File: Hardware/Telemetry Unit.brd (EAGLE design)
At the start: 50.8 x 63.5 mm, 56 parts, among them IC1 MEGA128-A, IC2 FT232RL, J2 503182-1852, J3 10118193-0001LF, Q1 10MHz, U1 MPL3115A2, U2 AP65111A, U3 LSM6DS3

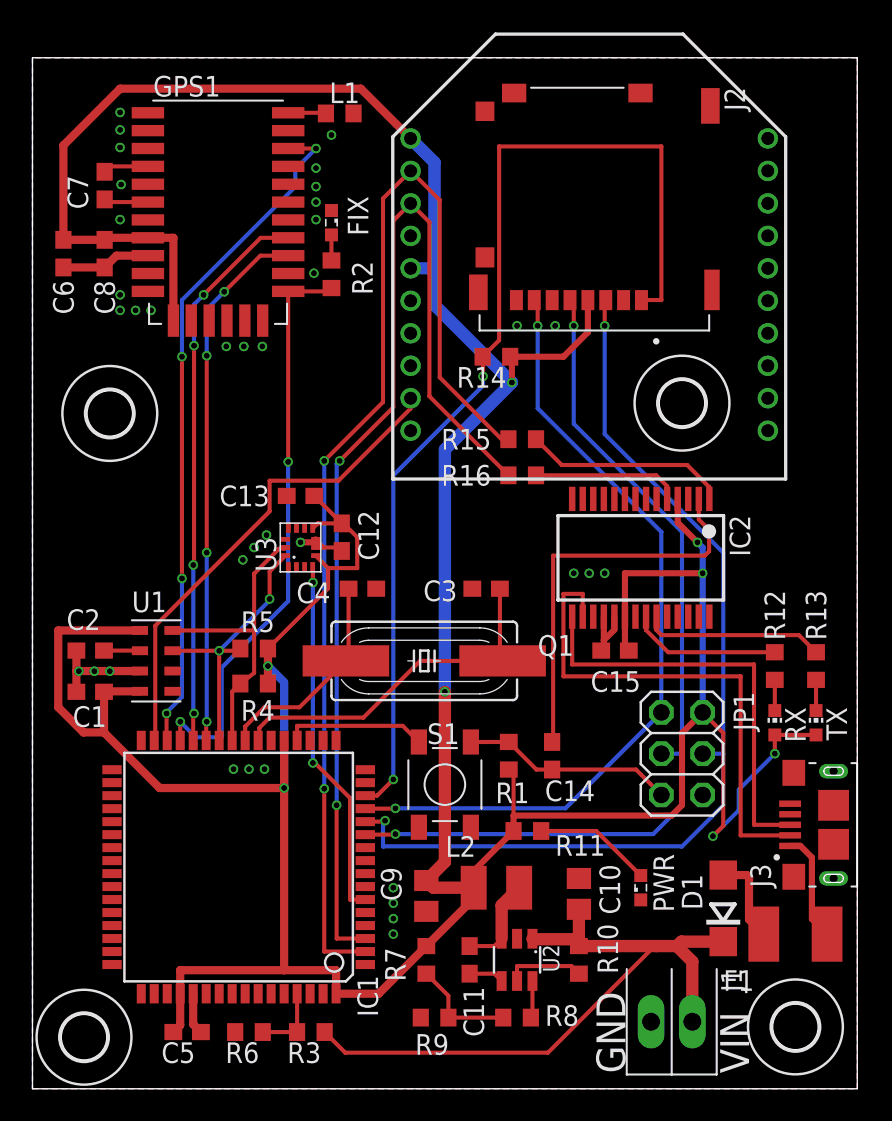
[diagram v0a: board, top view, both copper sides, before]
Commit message: Most minor updates and some rerouting
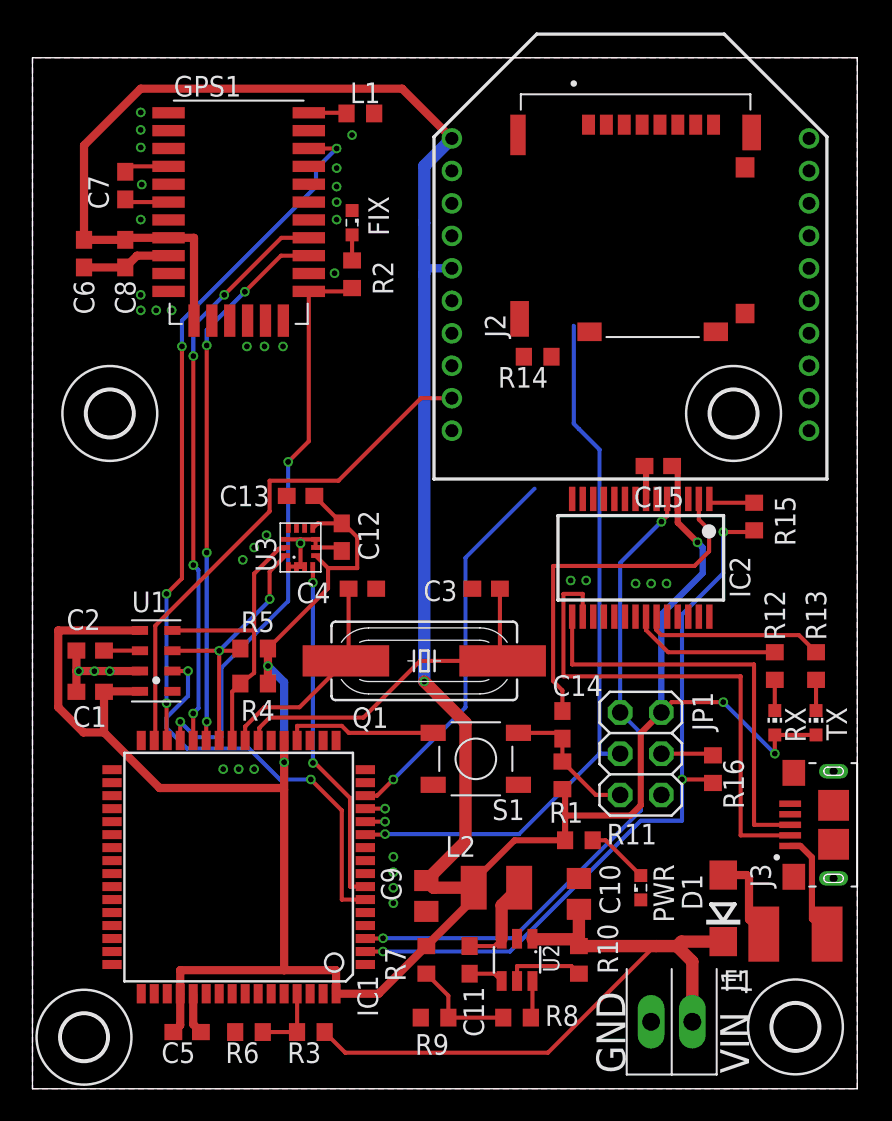
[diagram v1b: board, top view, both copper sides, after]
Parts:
- R11, R2: value 470 -> 1k
- R16: value 10k -> 330
- moved R16 21.6 mm to (41.9, 19.7), turned to 270 degrees
- moved R15 15.1 mm to (44.5, 35.2), turned to 270 degrees
- moved C15 11.7 mm to (38.5, 38.4)
- moved R1 3.52 mm to (32.6, 19.3)
- moved U$3 3.24 mm to (43.2, 41.6)
- moved R11 3.23 mm to (33.7, 15.3)
- moved J2 3.18 mm to (37.1, 53.0), turned to 0 degrees
- moved JP1 2.54 mm to (37.5, 20.6)
- moved R14 2.54 mm to (31.1, 45.1)
- moved XB1 2.54 mm to (36.8, 49.5)
- moved S1 2.48 mm to (27.3, 20.3), turned to 180 degrees
- moved C14 2.01 mm to (32.6, 22.4)
- moved L1 1.27 mm to (20.2, 60.1)
- moved C6 1.27 mm to (3.17, 51.4)
- moved C7 1.27 mm to (5.71, 55.6)
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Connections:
- removed net N$21: IC2.5, R16.1
- removed net RST2: C14.2, JP1.5, R1.2, S1.P$4
- removed net RX0: IC1.2, R15.2, XB1.2
- removed net TX0: IC1.3, R16.2, XB1.3
- new net ALT_INT: IC1.6, U1.6
- new net PDI: JP1.4, R16.1
- new net RX0/PDI: IC1.2, R15.2, R16.2, XB1.2
- new net TX0/PDO: IC1.3, IC2.5, JP1.1, XB1.3
- net !RST: now also C14.2, JP1.5, R1.2, S1.P2@1, S1.P2@2; no longer S1.P$3
- net +3V3: no longer IC2.20
- net ACCEL_INT: now also IC1.7; no longer IC1.6
- net CS_SD: now also J2.2; no longer J2.1
- net GND: now also S1.P1@1, S1.P1@2, U3.1, U3.12, U3.2, U3.3; no longer IC2.19, S1.P$1, S1.P$2
- net MISO: no longer JP1.1
- net MOSI: no longer JP1.4
- net V_USB: now also IC2.20
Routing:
- net RX0: track 72.1 -> 0.00 mm, vias 2 -> 0
- net TX0: track 68.2 -> 0.00 mm, vias 2 -> 0
- net MOSI: track 60.3 -> 1.22 mm, vias 2 -> 1
- net MISO: track 49.3 -> 1.22 mm, vias 2 -> 1
- net RX0/PDI: track 0.00 -> 45.6 mm, vias 0 -> 3
- net TX0/PDO: track 0.00 -> 41.1 mm, vias 0 -> 2
- net CS_SD: track 64.5 -> 23.7 mm, vias 2 -> 1
- net +3V3: track 271.6 -> 244.9 mm, vias 8 -> 6
- net ALT_INT: track 0.00 -> 24.9 mm, vias 0 -> 2
- net RST2: track 13.1 -> 0.00 mm
- net SCK: track 55.5 -> 44.8 mm, vias 2 -> 1
- net N$20: track 12.6 -> 3.00 mm
- net !RST: track 8.81 -> 18.1 mm
- net N$21: track 9.14 -> 0.00 mm
- net N$14: track 7.27 -> 3.86 mm
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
